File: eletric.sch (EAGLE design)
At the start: 14 parts, among them IC1 TINY26M

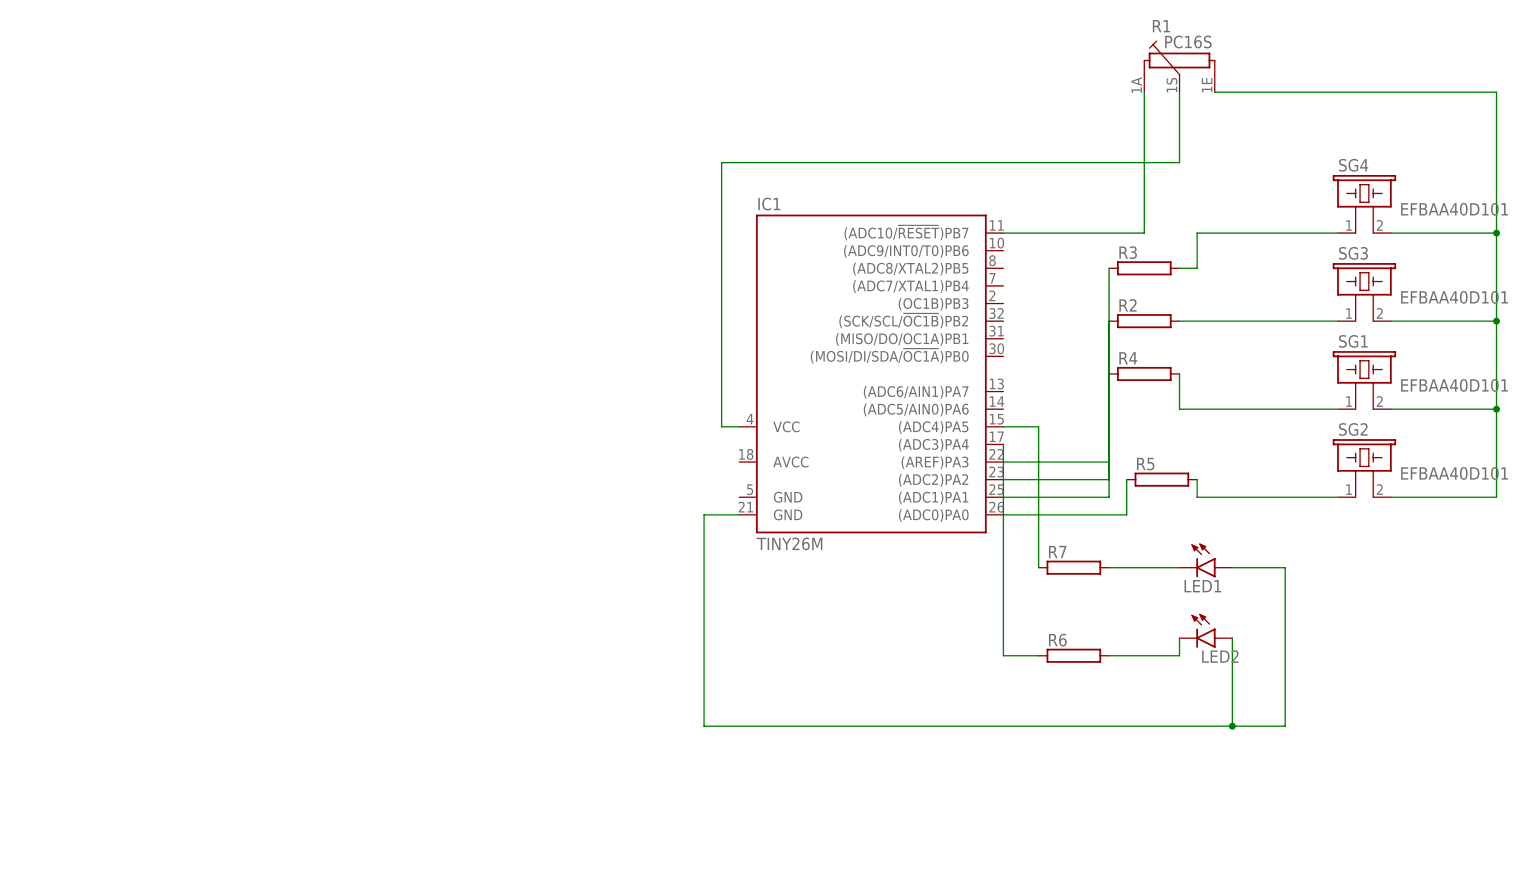
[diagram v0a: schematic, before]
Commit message: improve logical circuit
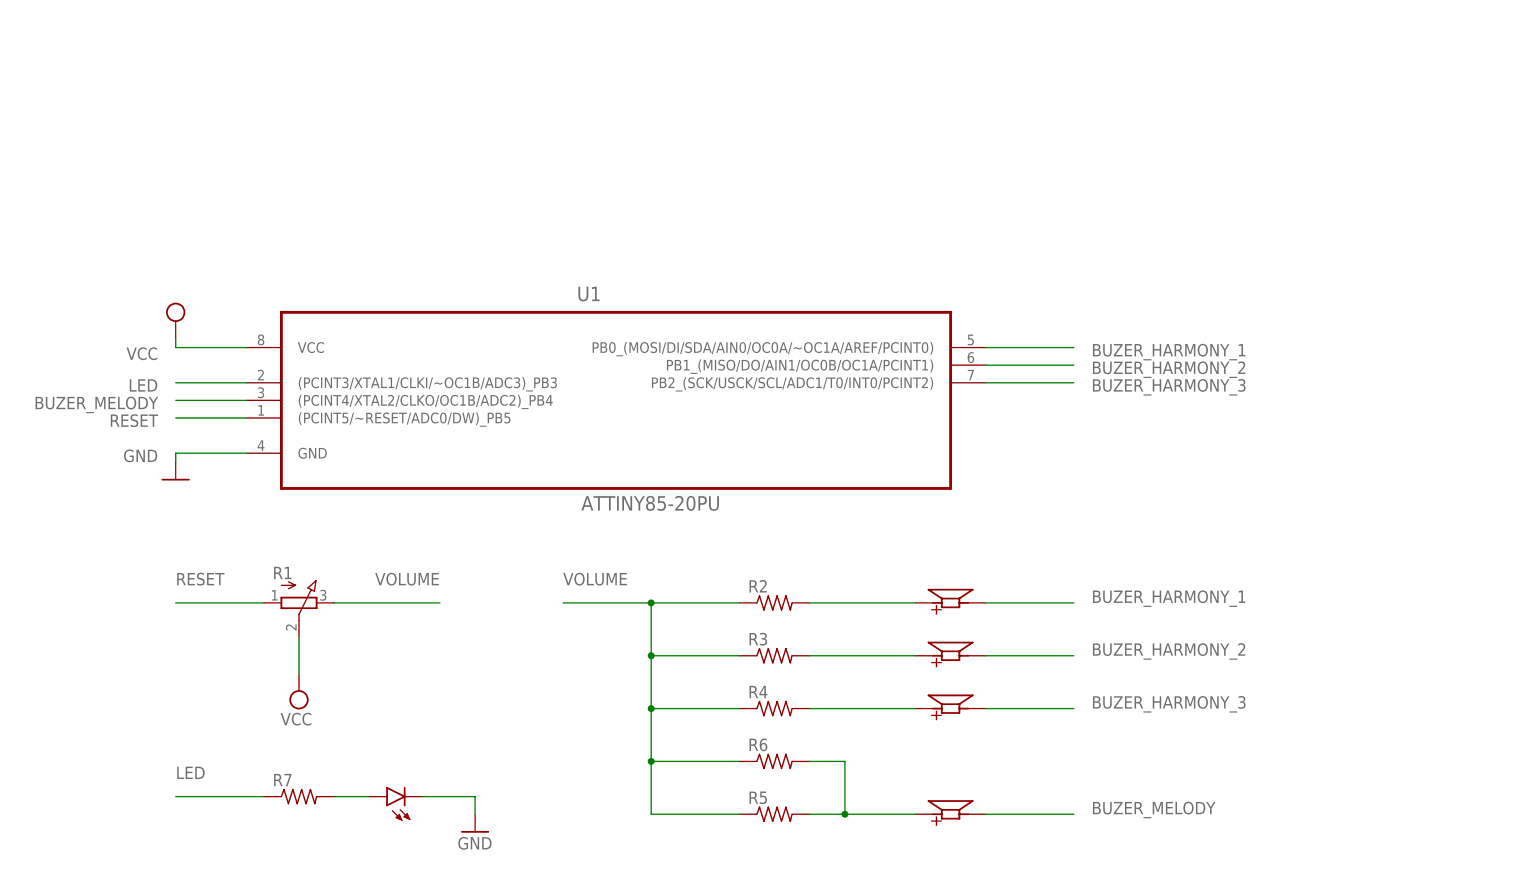
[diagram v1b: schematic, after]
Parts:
- removed IC1: TINY26M, atmel:TINY26M
- removed LED1: (no value), led:LED5MM
- removed SG1, SG2, SG3, SG4: EFBAA40D101, buzzer:EFBAA40D101
- added LS1, LS2, LS3, LS4: CMT-8530S-SMT, CMT-8530S-SMT:CMT-8530S-SMT
- added U1: ATTINY85-20PU, ATTINY85-20PU:ATTINY85-20PU
- R1: value PC16S -> (none); device piher:PC16S -> pot:3RP/1610N
- R2, R3, R4, R5, R6, R7: device resistor-power:RAC01 -> rcl:R-US_R0805
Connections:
- removed net N$1: R1.1E, SG1.2, SG2.2, SG3.2, SG4.2
- removed net N$10: IC1.(ADC2)PA2, R2.1
- removed net N$11: IC1.(AREF)PA3, R3.1
- removed net N$12: LED1.C, R7.2
- removed net N$13: LED2.C, R6.2
- removed net N$14: IC1.(ADC3)PA4, R6.1
- removed net N$15: IC1.(ADC4)PA5, R7.1
- removed net N$16: IC1.GND@1, LED1.A, LED2.A
- removed net N$7: R2.2, SG3.1
- removed net N$8: IC1.(ADC0)PA0, R5.1
- removed net N$9: IC1.(ADC1)PA1, R4.1
- new net BUZER_HARMONY_1: LS2.N, U1.PB0_(MOSI/DI/SDA/AIN0/OC0A/~OC1A/AREF/PCINT0)
- new net BUZER_HARMONY_2: LS4.N, U1.PB1_(MISO/DO/AIN1/OC0B/OC1A/PCINT1)
- new net BUZER_HARMONY_3: LS3.N, U1.PB2_(SCK/USCK/SCL/ADC1/T0/INT0/PCINT2)
- new net BUZER_MELODY: LS1.N, U1.(PCINT4/XTAL2/CLKO/OC1B/ADC2)_PB4
- new net GND: LED2.C, U1.GND
- new net LED: R7.1, U1.(PCINT3/XTAL1/CLKI/~OC1B/ADC3)_PB3
- new net RESET: R1.A, U1.(PCINT5/~RESET/ADC0/DW)_PB5
- new net VCC: R1.S, U1.VCC
- new net VOLUME: R1.E, R2.1, R3.1, R4.1, R5.1, R6.1
- net N$2: now also LS4.P, R3.2; no longer IC1.VCC, R1.1S
- net N$3: now also LS2.P, R2.2; no longer IC1.(ADC10/!RESET!)PB7, R1.1A
- net N$4: now also LS3.P, R4.2; no longer R3.2, SG4.1
- net N$5: now also LED2.A, R7.2; no longer R5.2, SG2.1
- net N$6: now also LS1.P, R5.2, R6.2; no longer R4.2, SG1.1
